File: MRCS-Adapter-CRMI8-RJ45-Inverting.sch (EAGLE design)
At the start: 17 parts, among them IC1 74LS540N, J1 RJ45, M1 MOUNTINGHOLE, M2 MOUNTINGHOLE

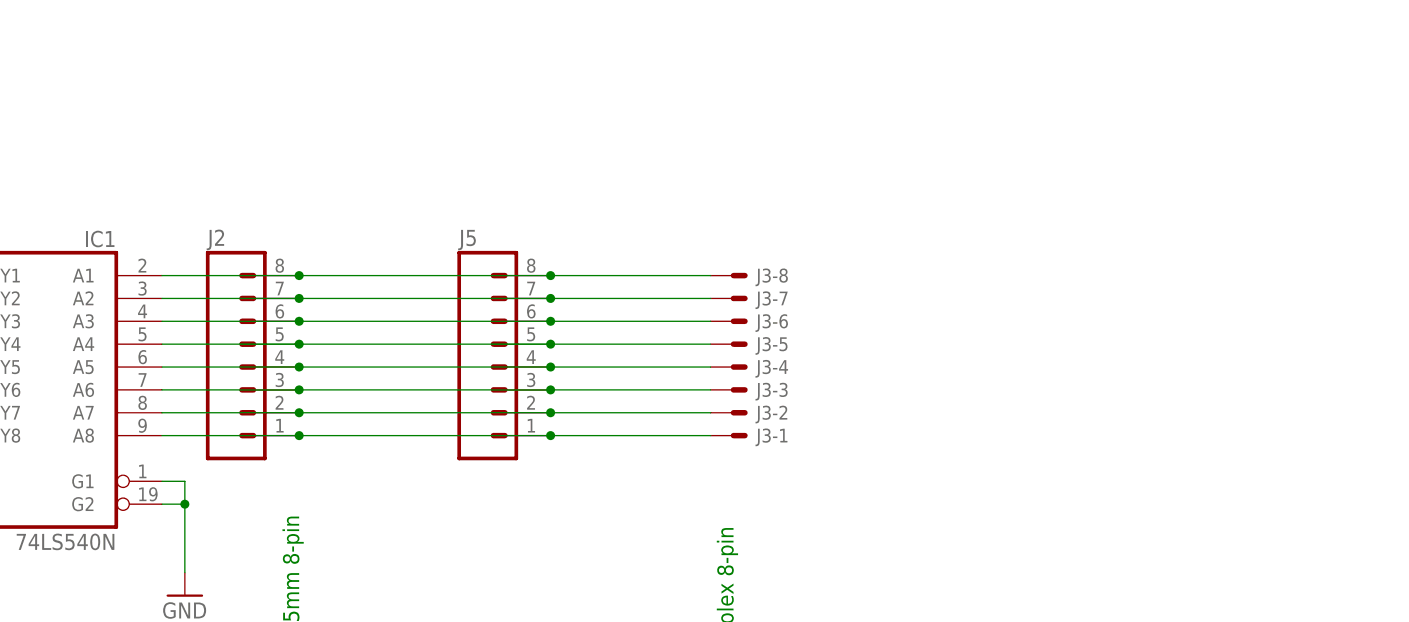
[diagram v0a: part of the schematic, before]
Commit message: various adjustments
minor board layout adjustments
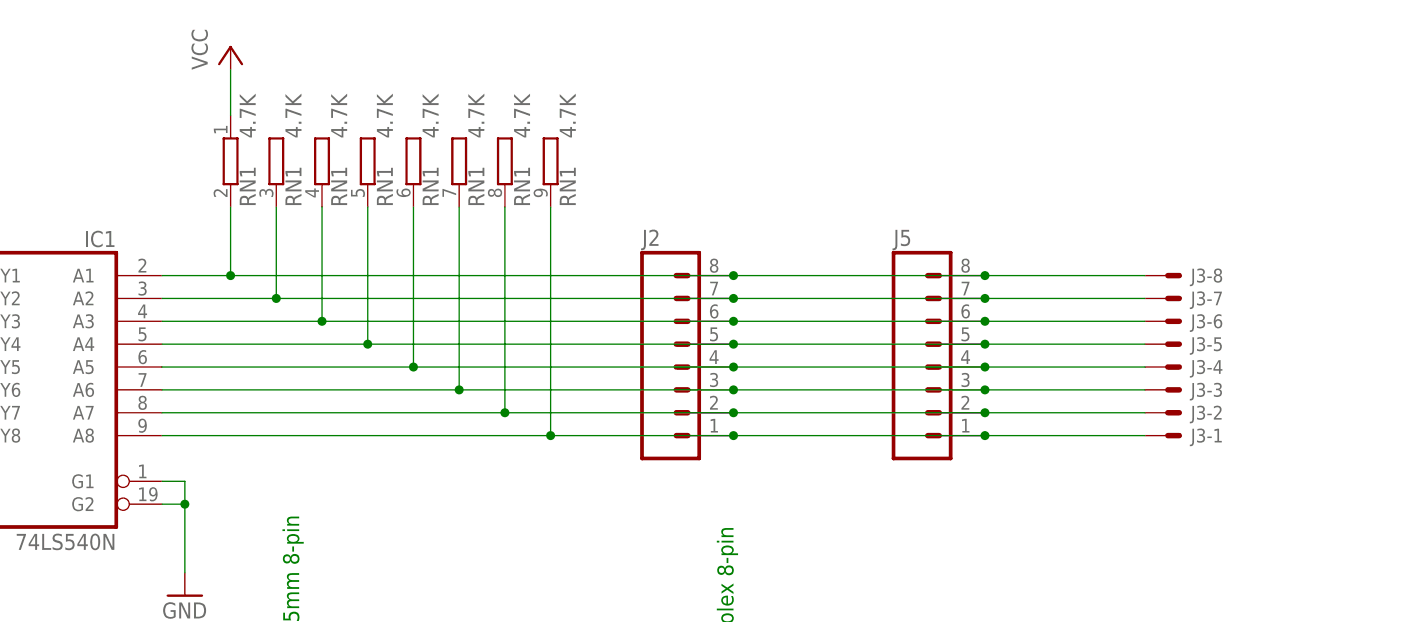
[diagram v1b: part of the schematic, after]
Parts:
- added RN1: 4.7K, resistor-sil:GE08RP
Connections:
- net L1: now also RN1H.2
- net L2: now also RN1G.2
- net L3: now also RN1F.2
- net L4: now also RN1E.2
- net L5: now also RN1D.2
- net L6: now also RN1C.2
- net L7: now also RN1B.2
- net L8: now also RN1A.2
- net VCC: now also RN1A.1
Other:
- moved on the sheet: J2, J3-1, J3-2, J3-3, J3-4, J3-5, J3-6, J3-7, J3-8, J5
